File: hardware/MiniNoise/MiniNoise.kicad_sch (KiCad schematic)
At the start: 16 parts, among them U1 TL072

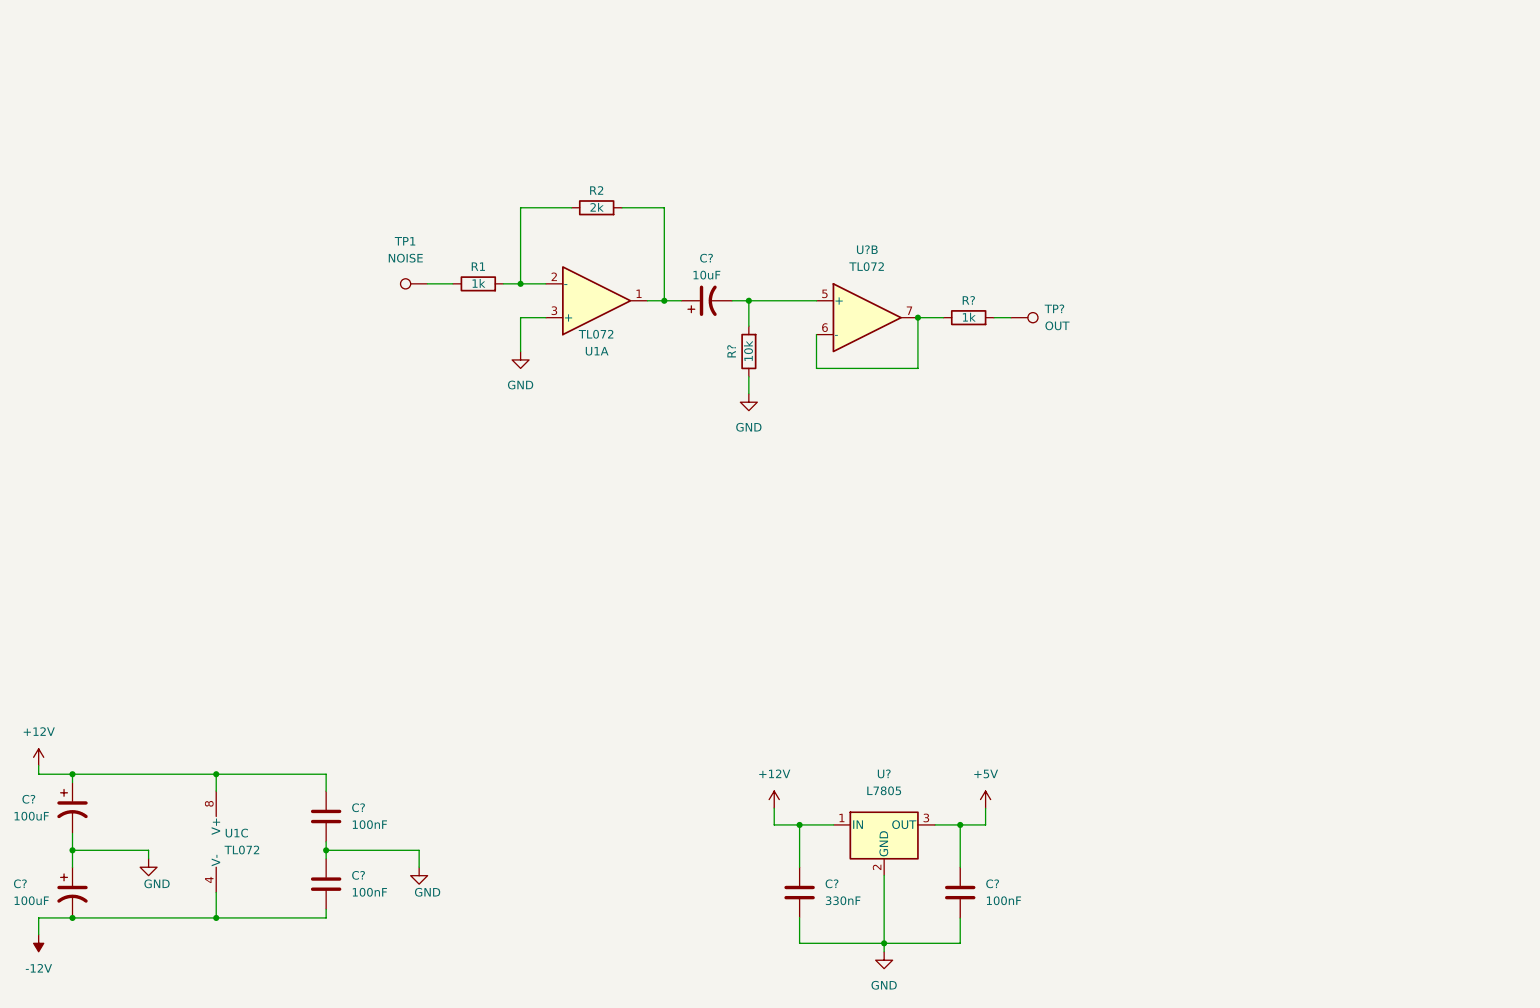
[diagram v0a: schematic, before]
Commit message: Added circuit
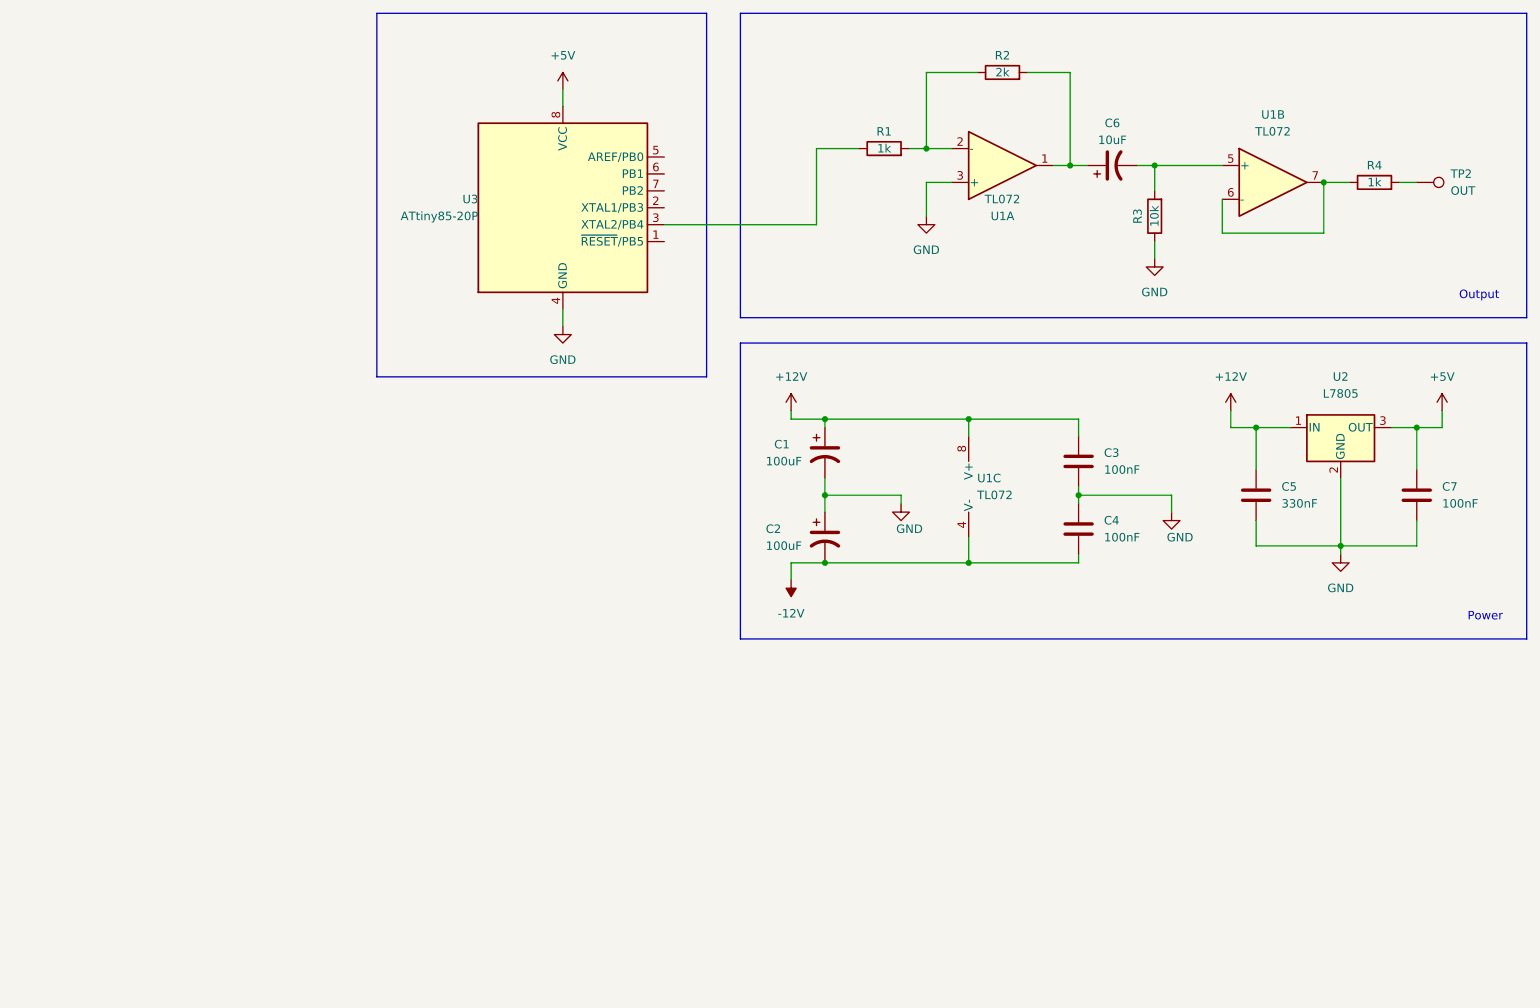
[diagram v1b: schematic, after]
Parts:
- removed TP1: NOISE, symbol Connector:TestPoint
- added U3: ATtiny85-20P, Package_DIP:DIP-8_W7.62mm, symbol MCU_Microchip_ATtiny:ATtiny85-20P
- gave numbers to parts that had none: 12
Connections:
- net +5V: now also U3.8 (VCC)
- net GND: now also U3.4 (GND)
- net at R1.1: now also U3.3 (XTAL2/PB4)
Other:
- note added: "Output"
- note added: "Power"
- moved on the sheet: C1, C2, C3, C4, C5, C6, C7, R1, R2, R3, R4, TP2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
